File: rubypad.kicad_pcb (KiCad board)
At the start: 2 copper layers, 65 x 77.5 mm, 32 parts, among them J1 HRO-TYPE-C, SW1 SW_Push, SW2 RotaryEncoder_Switch, U1 ATmega32U4-A, Y1 16MHz

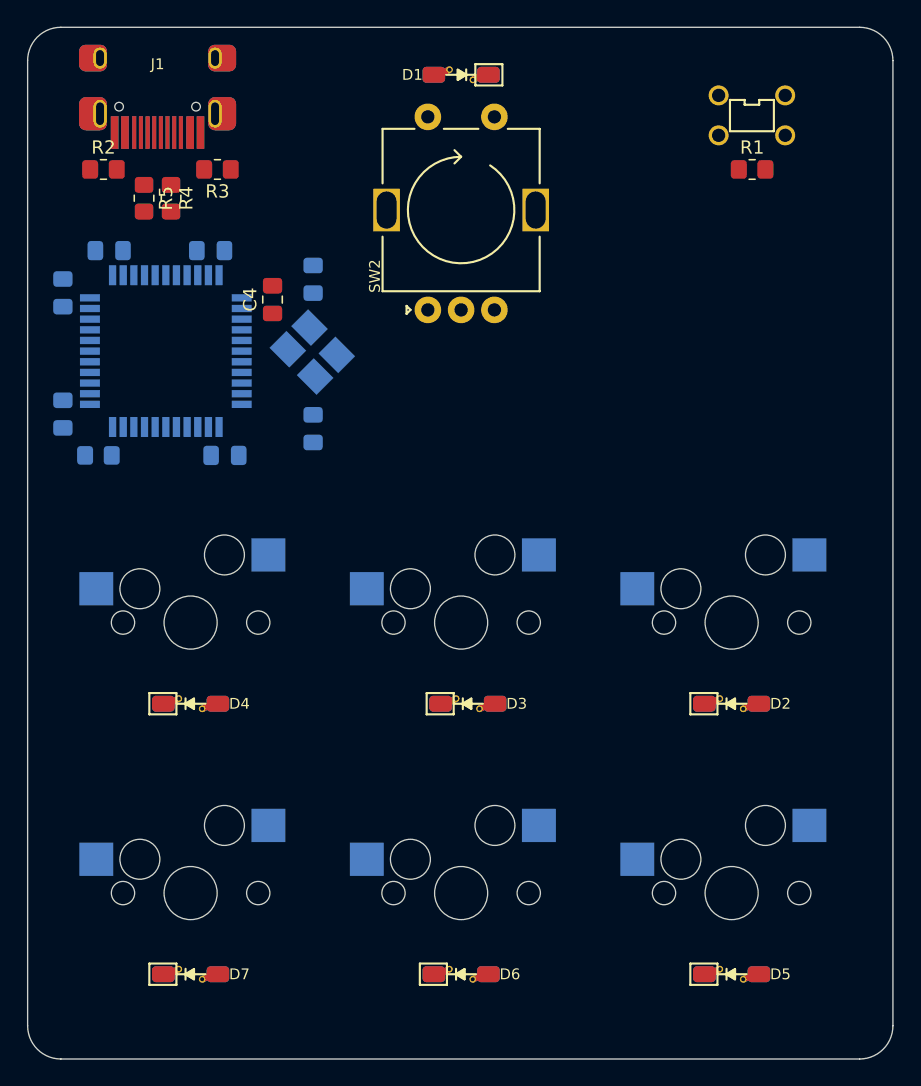
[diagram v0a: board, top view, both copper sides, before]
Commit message: changes and complete
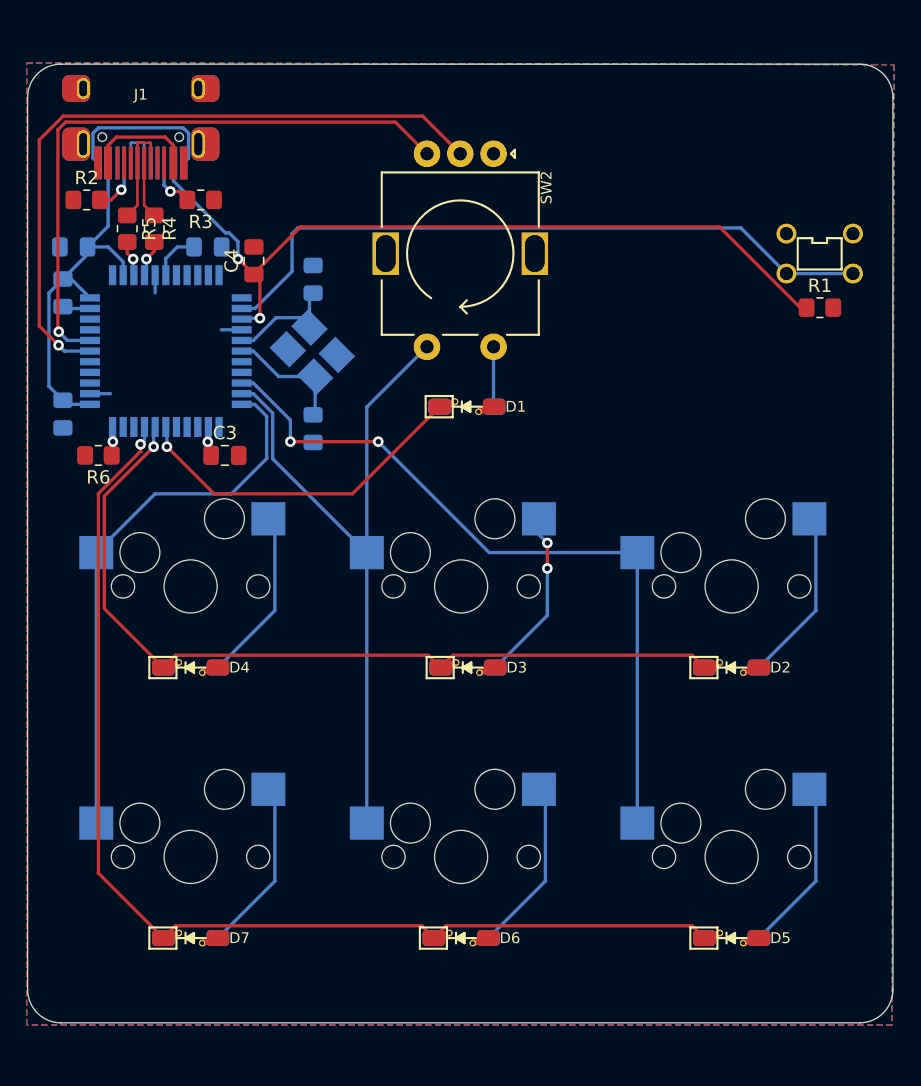
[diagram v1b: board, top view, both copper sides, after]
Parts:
- C3, R6: moved to F.Cu
- moved D1 24.9 mm to (68.0, 61.0), turned to 0 degrees
- moved R1 11.6 mm to (94.5, 53.6)
- moved SW1 11.6 mm to (94.5, 49.5)
- moved SW2 3.27 mm to (67.5, 49.5), turned to -90 degrees
- moved C4 3.23 mm to (52.0, 50.0)
- moved D5 2.72 mm to (87.9, 100.9)
- moved D6 2.72 mm to (67.6, 100.9)
- moved D7 2.72 mm to (47.2, 100.9)
- moved MX4 2.72 mm to (87.9, 94.8)
- moved MX5 2.72 mm to (67.6, 94.8)
- moved MX6 2.72 mm to (47.2, 94.8)
- moved D2 2.72 mm to (87.9, 80.6)
- moved D3 2.72 mm to (68.1, 80.6)
- moved D4 2.72 mm to (47.2, 80.6)
- moved MX1 2.72 mm to (87.9, 74.5)
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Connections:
- U1 pad 20: unconnected-(U1-Pad20) -> col0
- U1 pad 21: unconnected-(U1-Pad21) -> col1
- U1 pad 22: unconnected-(U1-Pad22) -> col2
- U1 pad 28: unconnected-(U1-Pad28) -> row0
- U1 pad 29: col0 -> row1
- U1 pad 30: col1 -> row2
- U1 pad 31: col2 -> unconnected-(U1-Pad31)
- U1 pad 38: unconnected-(U1-Pad38) -> encA
- U1 pad 39: unconnected-(U1-Pad39) -> encC
- U1 pad 40: unconnected-(U1-Pad40) -> encB
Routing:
- net VCC: track 0.00 -> 100.8 mm, vias 0 -> 3
- net row2: track 0.00 -> 84.0 mm, vias 0 -> 1
- net row1: track 0.00 -> 63.7 mm, vias 0 -> 1
- net col0: track 0.00 -> 56.3 mm, vias 0 -> 2
- net col1: track 0.00 -> 54.0 mm
- net encC: track 0.00 -> 52.1 mm, vias 0 -> 1
- net Net-(R1-Pad2): track 0.00 -> 51.5 mm
- net encB: track 0.00 -> 46.8 mm, vias 0 -> 1
- net col2: track 0.00 -> 41.5 mm
- net row0: track 0.00 -> 26.2 mm, vias 0 -> 1
- net GND: track 0.00 -> 18.8 mm
- net Net-(D6-Pad2): track 0.00 -> 13.2 mm
- net Net-(D7-Pad2): track 0.00 -> 13.2 mm
- net Net-(D5-Pad2): track 0.00 -> 13.2 mm
- net Net-(D4-Pad2): track 0.00 -> 13.2 mm
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- added copper zone on B.Cu, net GND
- added copper zone on F.Cu, net GND
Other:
- board size 65 x 77.5 mm -> 65 x 72 mm
